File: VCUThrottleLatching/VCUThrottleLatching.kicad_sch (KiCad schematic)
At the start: 9 parts, among them J1 B12B-PH-K-S:JST_B12B-PH-K-S, U1 IRLML2060TRPBF, U2 IRLML2060TRPBF

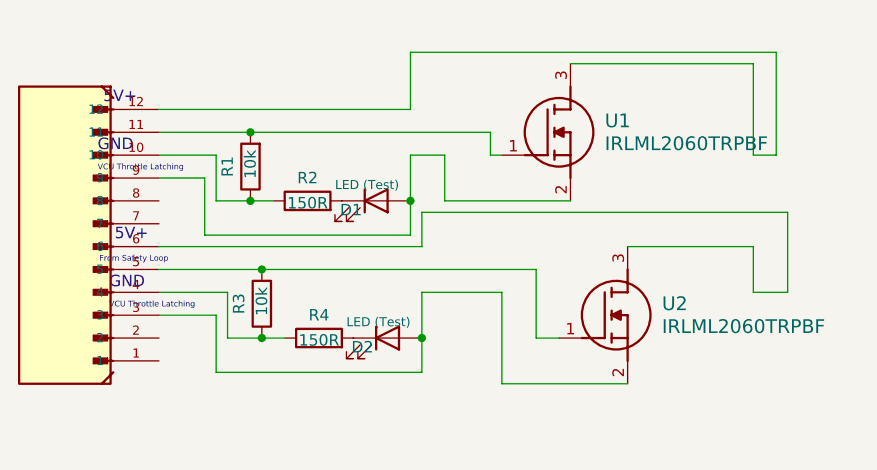
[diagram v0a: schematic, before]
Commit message: documentation
documentation
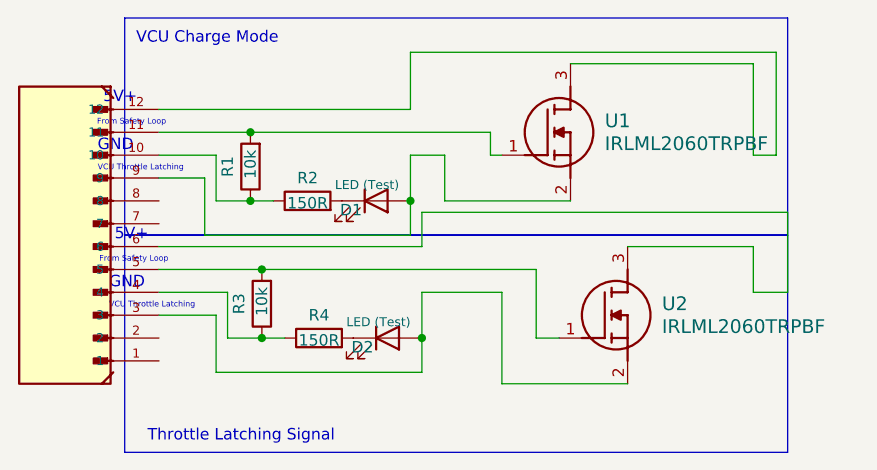
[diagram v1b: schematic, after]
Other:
- note added: "Throttle Latching Signal"
- note added: "VCU Charge Mode"
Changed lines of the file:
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@@
 	(generator_version "9.0")
 	(paper "A4")
+	(rectangle
+		(start 43.18 53.34)
+		(end 116.84 77.47)
+		(stroke
+			(width 0)
+			(type default)
+		)
+		(fill
+			(type none)
+		)
+	)
+	(rectangle
+		(start 43.18 77.47)
+		(end 116.84 101.6)
+		(stroke
+			(width 0)
+			(type default)
+		)
+		(fill
+			(type none)
+		)
+	)
+	(text "VCU Charge Mode \n\n"
+		(exclude_from_sim no)
+		(at 44.45 58.42 0)
+		(effects
+			(font
+				(face "KiCad Font")
+				(size 1.27 1.27)
+			)
+			(justify left bottom)
+		)
+	)
 	(text "VCU Throttle Latching\n"
 		(exclude_from_sim no)
@@
 			)
 		)
+	)
+	(text "Throttle Latching Signal\n\n"
+		(exclude_from_sim no)
+		(at 45.72 102.616 0)
+		(effects
+			(font
+				(face "KiCad Font")
+				(size 1.27 1.27)
+			)
+			(justify left bottom)
+		)
+	)
+	(text "From Safety Loop\n"
+		(exclude_from_sim no)
+		(at 43.942 65.024 0)
+		(effects
+			(font
+				(size 0.635 0.635)
+			)
+		)
